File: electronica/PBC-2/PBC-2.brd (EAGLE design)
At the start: 210 x 196.1 mm, 9 parts

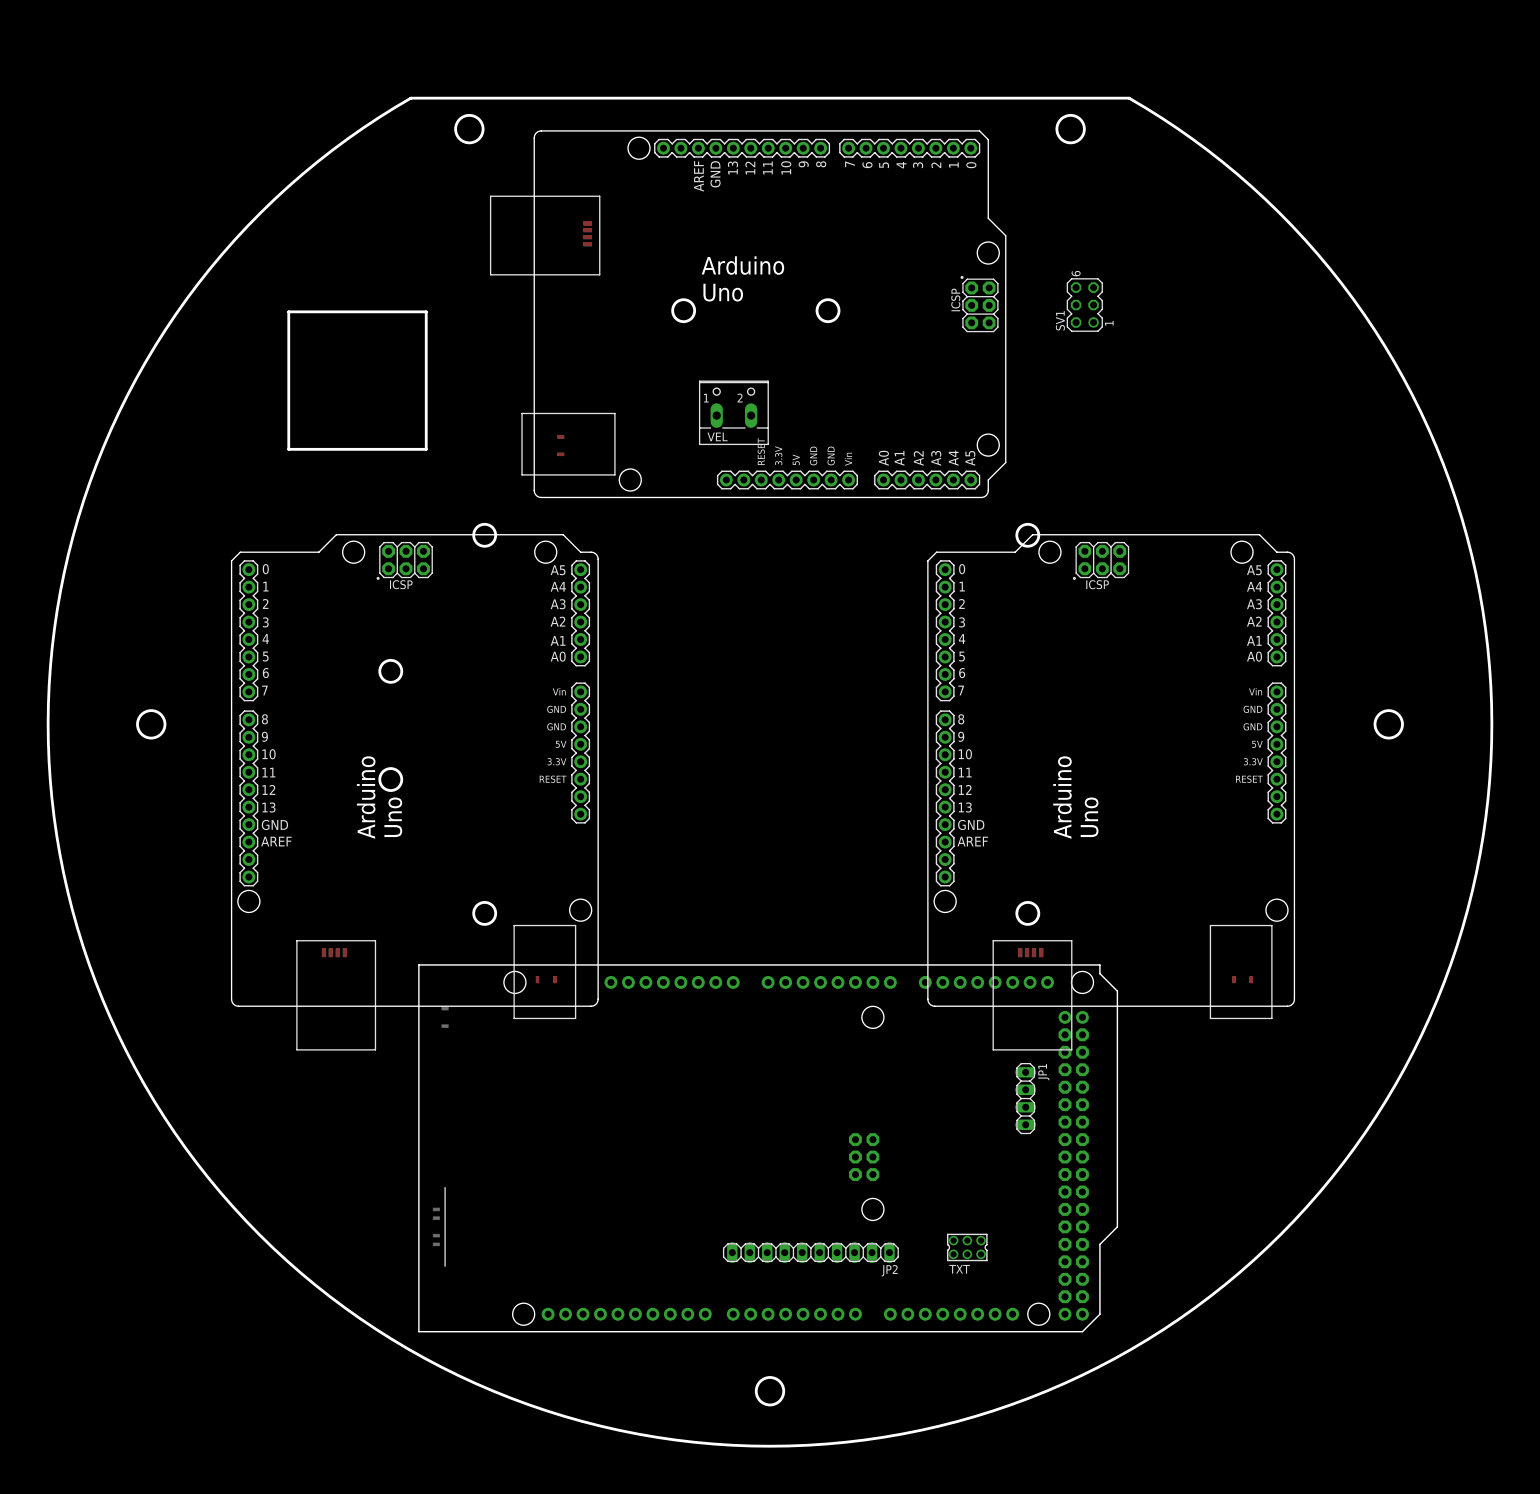
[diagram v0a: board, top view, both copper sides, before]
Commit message: fin pcb-2
fin pcb-2
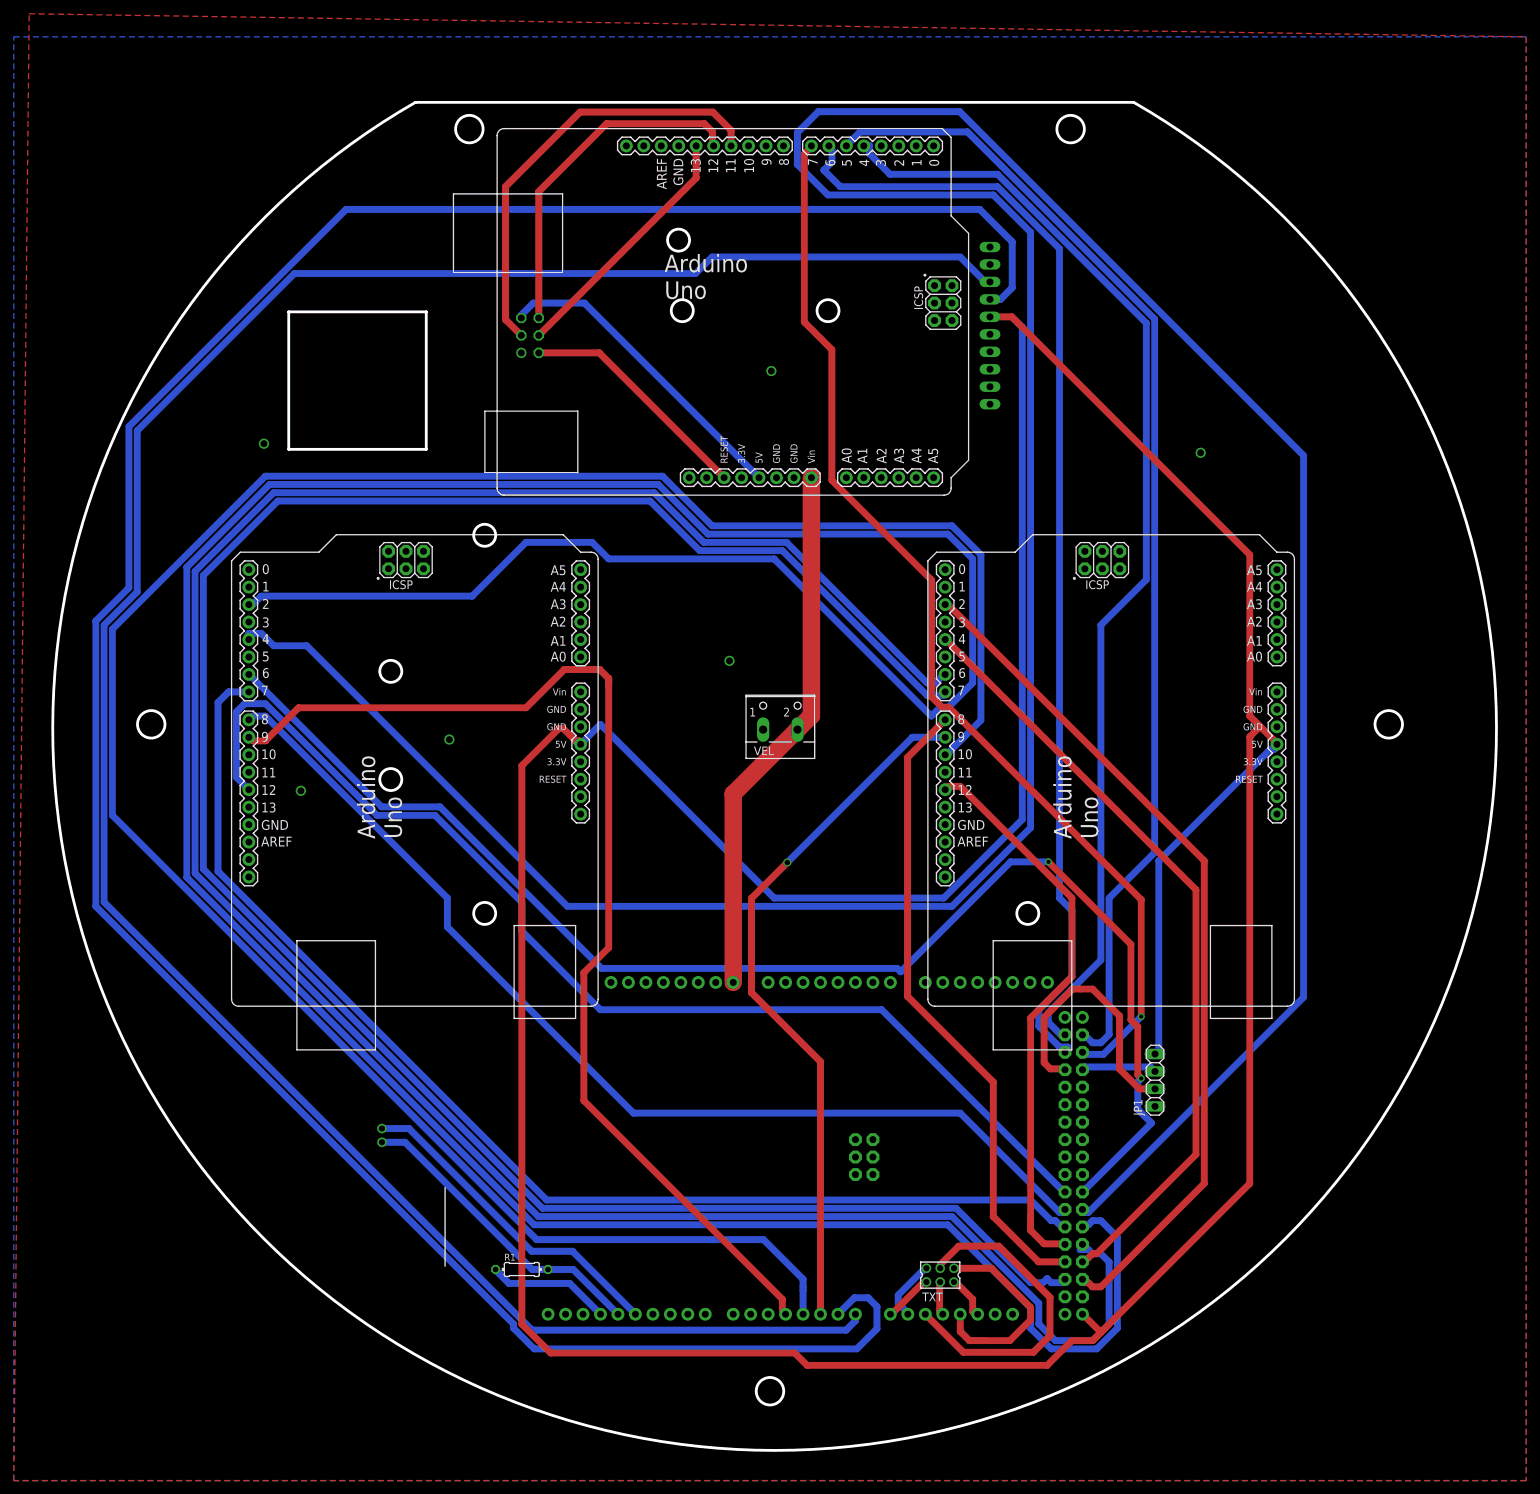
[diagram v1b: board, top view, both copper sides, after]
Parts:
- added BTN: (no value), con-garry:332-02
- added R1: (no value), eagle-ltspice:0204/7
- moved JP2 137.3 mm to (32.0, 58.0), flipped to the bottom, turned to 270 degrees
- moved SV1 80.8 mm to (-34.9, 56.6), flipped to the bottom
- moved VEL 46.2 mm to (1.50, 0.51)
- moved JP1 19.0 mm to (56.0, -51.8), turned to 90 degrees
- moved TXT 5.63 mm to (24.8, -80.1)
- moved UNO 5.41 mm to (-39.7, 33.3)
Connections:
- new net S$1: BTN.2, MEGA.12
- new net S$2: BTN.1, MEGA.13, R1.2
- new net S$3: MEGA.GND, R1.1
- net +5V: now also MEGA.5V..
- net RX-XBEE: no longer JP2.4
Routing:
- net +5V: track 0.00 -> 571.3 mm
- net M1INAL: track 0.00 -> 494.9 mm
- net M1INBL: track 0.00 -> 484.8 mm
- net RX-XBEE: track 0.00 -> 378.8 mm
- net M1ENR: track 0.00 -> 348.5 mm
- net TX-XBEE: track 0.00 -> 344.1 mm
- net M2PWMR: track 0.00 -> 332.2 mm
- net M2INAR: track 0.00 -> 318.2 mm
- net M1ENL: track 0.00 -> 199.7 mm, vias 0 -> 2
- net M2INAL: track 0.00 -> 174.6 mm
- net PIXY3: track 0.00 -> 168.7 mm
- net PIXY2: track 0.00 -> 165.6 mm
- net M2ENL: track 0.00 -> 165.0 mm
- net M1PWML: track 0.00 -> 164.5 mm
- net PIXY4: track 0.00 -> 163.3 mm
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- added copper zone on layer 1, net GND
- added copper zone on layer 16, net GND
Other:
- outline, holes or cut-outs redrawn
- board text added: "C:/Users/carlos hugo/Desktop/github/L16/electronica/PBC-2/InteliRobot.bmp"
- board text added: "C:/Users/carlos hugo/Desktop/github/L16/electronica/PBC-2/yoHagoRobots.bmp"
- board text added: "InteliRobot"

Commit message: ELECTRONICA
FIN DE LOS DISEÑOS
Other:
- board text removed: "C:/Users/carlos hugo/Desktop/github/L16/electronica/PBC-2/yoHagoRobots.bmp"
